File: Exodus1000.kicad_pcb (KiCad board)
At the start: 2 copper layers, 81.3 x 132.1 mm, 35 parts, among them J1 ARJ-169, M1 ET60S-02-24-02-X-VP-GP, M2 ET60S-02-24-02-X-VP-GP, M3 ET60S-02-24-02-X-VP-GP, M4 ET60S-02-24-02-X-VP-GP, U1 TM4C1294NCPDTGOOD, U2 93LCxxB, U3 FT232H, U4 TUSB4041I, U5 FSUSB42UMX, Y1 Crystal_GND24, Y2 Crystal

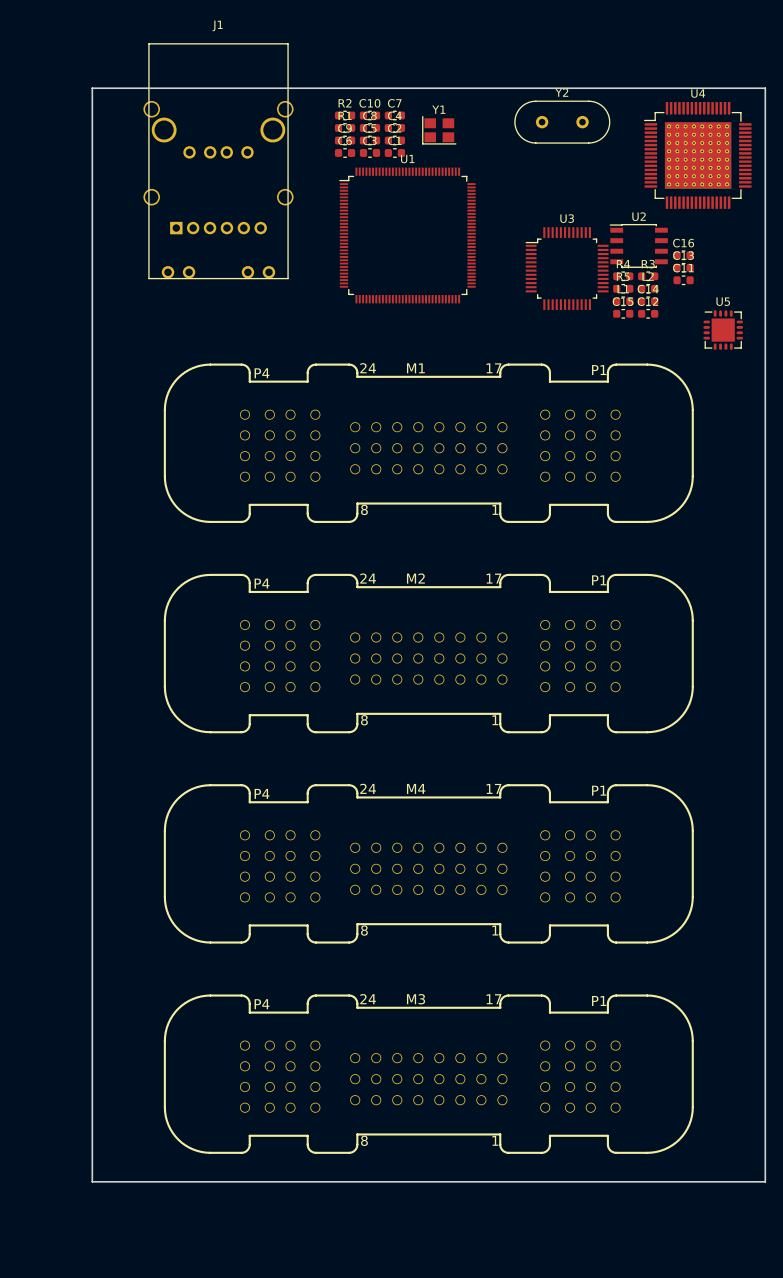
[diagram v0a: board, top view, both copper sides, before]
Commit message: layout stuff
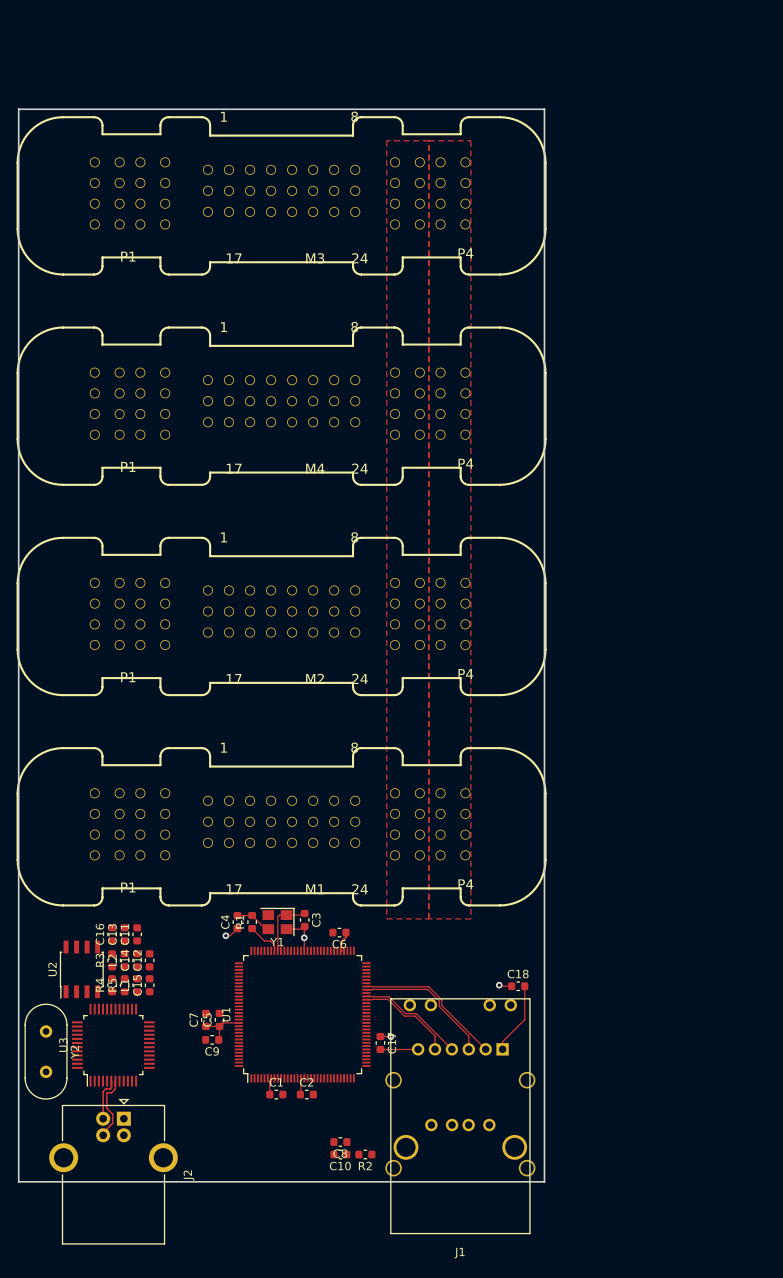
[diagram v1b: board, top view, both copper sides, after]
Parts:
- removed U4: TUSB4041I, Package_QFP:HTQFP-64-1EP_10x10mm_P0.5mm_EP8x8mm_Mask4.4x4.4mm_ThermalVias
- removed U5: FSUSB42UMX, Package_DFN_QFN:MLPQ-16-1EP_4x4mm_P0.65mm_EP2.8x2.8mm
- added C17: C_Small, Capacitor_SMD:C_0603_1608Metric, F.Cu at (118.6, 140.7)
- added C18: C_Small, Capacitor_SMD:C_0603_1608Metric, F.Cu at (135.3, 133.9)
- added J2: USB_B, Connector_USB:USB_B_OST_USB-B1HSxx_Horizontal, F.Cu at (87.6, 149.9)
- moved J1 131.2 mm to (128.3, 155.8), turned to 0 degrees
- moved C10 125.5 mm to (113.8, 154.2), turned to 180 degrees
- moved R2 125.5 mm to (116.8, 154.2), turned to 180 degrees
- moved Y2 125.1 mm to (78.2, 139.3), turned to 270 degrees
- moved C8 122.5 mm to (113.8, 152.7), turned to 180 degrees
- moved C2 115.7 mm to (109.7, 146.9)
- moved C1 114.6 mm to (106.0, 146.9)
- moved C7 111.6 mm to (97.5, 137.9), turned to 90 degrees
- moved U2 110.3 mm to (82.5, 131.8), turned to 90 degrees
- moved C9 109.8 mm to (98.3, 140.3), turned to 180 degrees
- moved U3 108.6 mm to (86.4, 141.0), turned to 90 degrees
- moved M3 108.2 mm to (106.7, 38.1), turned to 180 degrees
- moved C5 107.7 mm to (99.2, 137.9), turned to 90 degrees
- moved C16 107.2 mm to (86.2, 127.6), turned to 90 degrees
- moved R4 105.6 mm to (86.2, 133.7), turned to 90 degrees
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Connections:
- J1 pad P2: Net-(J1-PadP2) -> /TM4C129/ETH_TXO_P
- J1 pad P3: Net-(J1-PadP3) -> /TM4C129/ETH_TXO_N
- J1 pad P4: Net-(J1-PadP4) -> /TM4C129/ETH_RXI_P
- J1 pad P5: Net-(J1-PadP5) -> /TM4C129/ETH_RXI_N
- J1 pad SH1: Net-(J1-PadSH1) -> GND
- J1 pad SH2: Net-(J1-PadSH1) -> GND
- J1 pad SH3: Net-(J1-PadSH1) -> GND
- J1 pad SH4: Net-(J1-PadSH1) -> GND
- J1 pad SH5: Net-(J1-PadSH1) -> GND
- J1 pad SH6: Net-(J1-PadSH1) -> GND
- J1 pad U2: Net-(J1-PadU2) -> /TM4C129/USB_D_N
- J1 pad U3: Net-(J1-PadU3) -> /TM4C129/USB_D_P
- J1 pad U4: Net-(J1-PadU4) -> GND
- M1 pad P1-1: Net-(M1-PadP1-1) -> GND
- M1 pad P1-2: Net-(M1-PadP1-2) -> GND
- M1 pad P1-3: Net-(M1-PadP1-3) -> GND
- M1 pad P1-4: Net-(M1-PadP1-4) -> GND
- M1 pad P1-5: Net-(M1-PadP1-5) -> GND
- M1 pad P1-6: Net-(M1-PadP1-6) -> GND
- M1 pad P1-7: Net-(M1-PadP1-7) -> GND
- M1 pad P1-8: Net-(M1-PadP1-8) -> GND
- M1 pad P2-1: Net-(M1-PadP2-1) -> +BATT
- M1 pad P2-2: Net-(M1-PadP2-2) -> +BATT
- M1 pad P2-3: Net-(M1-PadP2-3) -> +BATT
- M1 pad P2-4: Net-(M1-PadP2-4) -> +BATT
- M1 pad P2-5: Net-(M1-PadP2-5) -> +BATT
- M1 pad P2-6: Net-(M1-PadP2-6) -> +BATT
- M1 pad P2-7: Net-(M1-PadP2-7) -> +BATT
- M1 pad P2-8: Net-(M1-PadP2-8) -> +BATT
- M1 pad P3-1: Net-(M1-PadP3-1) -> +5V
- M1 pad P3-2: Net-(M1-PadP3-2) -> +5V
- M1 pad P3-3: Net-(M1-PadP3-3) -> +5V
- M1 pad P3-4: Net-(M1-PadP3-4) -> +5V
- M1 pad P3-5: Net-(M1-PadP3-5) -> +5V
- M1 pad P3-6: Net-(M1-PadP3-6) -> +5V
- M1 pad P3-7: Net-(M1-PadP3-7) -> +5V
- M1 pad P3-8: Net-(M1-PadP3-8) -> +5V
- M1 pad P4-1: Net-(M1-PadP4-1) -> +3V3
- M1 pad P4-2: Net-(M1-PadP4-2) -> +3V3
- M1 pad P4-3: Net-(M1-PadP4-3) -> +3V3
- M1 pad P4-4: Net-(M1-PadP4-4) -> +3V3
- M1 pad P4-5: Net-(M1-PadP4-5) -> +3V3
- M1 pad P4-6: Net-(M1-PadP4-6) -> +3V3
- M1 pad P4-7: Net-(M1-PadP4-7) -> +3V3
- M1 pad P4-8: Net-(M1-PadP4-8) -> +3V3
- M2 pad P1-1: Net-(M2-PadP1-1) -> GND
- M2 pad P1-2: Net-(M2-PadP1-2) -> GND
- M2 pad P1-3: Net-(M2-PadP1-3) -> GND
- M2 pad P1-4: Net-(M2-PadP1-4) -> GND
- M2 pad P1-5: Net-(M2-PadP1-5) -> GND
- M2 pad P1-6: Net-(M2-PadP1-6) -> GND
- M2 pad P1-7: Net-(M2-PadP1-7) -> GND
- M2 pad P1-8: Net-(M2-PadP1-8) -> GND
- M2 pad P2-1: Net-(M2-PadP2-1) -> +BATT
- M2 pad P2-2: Net-(M2-PadP2-2) -> +BATT
- M2 pad P2-3: Net-(M2-PadP2-3) -> +BATT
- M2 pad P2-4: Net-(M2-PadP2-4) -> +BATT
- M2 pad P2-5: Net-(M2-PadP2-5) -> +BATT
- M2 pad P2-6: Net-(M2-PadP2-6) -> +BATT
- M2 pad P2-7: Net-(M2-PadP2-7) -> +BATT
- M2 pad P2-8: Net-(M2-PadP2-8) -> +BATT
- M2 pad P3-1: Net-(M2-PadP3-1) -> +5V
- M2 pad P3-2: Net-(M2-PadP3-2) -> +5V
- M2 pad P3-3: Net-(M2-PadP3-3) -> +5V
- M2 pad P3-4: Net-(M2-PadP3-4) -> +5V
- M2 pad P3-5: Net-(M2-PadP3-5) -> +5V
- M2 pad P3-6: Net-(M2-PadP3-6) -> +5V
- M2 pad P3-7: Net-(M2-PadP3-7) -> +5V
- M2 pad P3-8: Net-(M2-PadP3-8) -> +5V
- M2 pad P4-1: Net-(M2-PadP4-1) -> +3V3
- M2 pad P4-2: Net-(M2-PadP4-2) -> +3V3
- M2 pad P4-3: Net-(M2-PadP4-3) -> +3V3
- M2 pad P4-4: Net-(M2-PadP4-4) -> +3V3
- M2 pad P4-5: Net-(M2-PadP4-5) -> +3V3
- M2 pad P4-6: Net-(M2-PadP4-6) -> +3V3
- M2 pad P4-7: Net-(M2-PadP4-7) -> +3V3
- M2 pad P4-8: Net-(M2-PadP4-8) -> +3V3
- M3 pad P1-1: Net-(M3-PadP1-1) -> GND
- M3 pad P1-2: Net-(M3-PadP1-2) -> GND
- M3 pad P1-3: Net-(M3-PadP1-3) -> GND
- M3 pad P1-4: Net-(M3-PadP1-4) -> GND
- M3 pad P1-5: Net-(M3-PadP1-5) -> GND
- M3 pad P1-6: Net-(M3-PadP1-6) -> GND
- M3 pad P1-7: Net-(M3-PadP1-7) -> GND
- M3 pad P1-8: Net-(M3-PadP1-8) -> GND
- M3 pad P2-1: Net-(M3-PadP2-1) -> +BATT
- M3 pad P2-2: Net-(M3-PadP2-2) -> +BATT
- M3 pad P2-3: Net-(M3-PadP2-3) -> +BATT
- M3 pad P2-4: Net-(M3-PadP2-4) -> +BATT
- M3 pad P2-5: Net-(M3-PadP2-5) -> +BATT
- M3 pad P2-6: Net-(M3-PadP2-6) -> +BATT
- M3 pad P2-7: Net-(M3-PadP2-7) -> +BATT
- M3 pad P2-8: Net-(M3-PadP2-8) -> +BATT
- M3 pad P3-1: Net-(M3-PadP3-1) -> +5V
- M3 pad P3-2: Net-(M3-PadP3-2) -> +5V
- M3 pad P3-3: Net-(M3-PadP3-3) -> +5V
- M3 pad P3-4: Net-(M3-PadP3-4) -> +5V
- M3 pad P3-5: Net-(M3-PadP3-5) -> +5V
- M3 pad P3-6: Net-(M3-PadP3-6) -> +5V
- M3 pad P3-7: Net-(M3-PadP3-7) -> +5V
- M3 pad P3-8: Net-(M3-PadP3-8) -> +5V
- M3 pad P4-1: Net-(M3-PadP4-1) -> +3V3
- M3 pad P4-2: Net-(M3-PadP4-2) -> +3V3
- M3 pad P4-3: Net-(M3-PadP4-3) -> +3V3
- M3 pad P4-4: Net-(M3-PadP4-4) -> +3V3
- M3 pad P4-5: Net-(M3-PadP4-5) -> +3V3
- M3 pad P4-6: Net-(M3-PadP4-6) -> +3V3
- M3 pad P4-7: Net-(M3-PadP4-7) -> +3V3
- M3 pad P4-8: Net-(M3-PadP4-8) -> +3V3
- M4 pad P1-1: Net-(M4-PadP1-1) -> GND
- M4 pad P1-2: Net-(M4-PadP1-2) -> GND
- M4 pad P1-3: Net-(M4-PadP1-3) -> GND
- M4 pad P1-4: Net-(M4-PadP1-4) -> GND
- M4 pad P1-5: Net-(M4-PadP1-5) -> GND
- M4 pad P1-6: Net-(M4-PadP1-6) -> GND
- M4 pad P1-7: Net-(M4-PadP1-7) -> GND
- M4 pad P1-8: Net-(M4-PadP1-8) -> GND
- M4 pad P2-1: Net-(M4-PadP2-1) -> +BATT
- M4 pad P2-2: Net-(M4-PadP2-2) -> +BATT
- M4 pad P2-3: Net-(M4-PadP2-3) -> +BATT
- M4 pad P2-4: Net-(M4-PadP2-4) -> +BATT
- M4 pad P2-5: Net-(M4-PadP2-5) -> +BATT
- M4 pad P2-6: Net-(M4-PadP2-6) -> +BATT
- M4 pad P2-7: Net-(M4-PadP2-7) -> +BATT
- M4 pad P2-8: Net-(M4-PadP2-8) -> +BATT
- M4 pad P3-1: Net-(M4-PadP3-1) -> +5V
- M4 pad P3-2: Net-(M4-PadP3-2) -> +5V
- M4 pad P3-3: Net-(M4-PadP3-3) -> +5V
- M4 pad P3-4: Net-(M4-PadP3-4) -> +5V
- M4 pad P3-5: Net-(M4-PadP3-5) -> +5V
- M4 pad P3-6: Net-(M4-PadP3-6) -> +5V
- M4 pad P3-7: Net-(M4-PadP3-7) -> +5V
- M4 pad P3-8: Net-(M4-PadP3-8) -> +5V
- M4 pad P4-1: Net-(M4-PadP4-1) -> +3V3
- M4 pad P4-2: Net-(M4-PadP4-2) -> +3V3
- M4 pad P4-3: Net-(M4-PadP4-3) -> +3V3
- M4 pad P4-4: Net-(M4-PadP4-4) -> +3V3
- M4 pad P4-5: Net-(M4-PadP4-5) -> +3V3
- M4 pad P4-6: Net-(M4-PadP4-6) -> +3V3
- M4 pad P4-7: Net-(M4-PadP4-7) -> +3V3
- M4 pad P4-8: Net-(M4-PadP4-8) -> +3V3
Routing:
- net /TM4C129/ETH_TXO_P: track 0.00 -> 18.0 mm
- net /TM4C129/ETH_TXO_N: track 0.00 -> 16.7 mm
- net /TM4C129/ETH_RXI_P: track 0.00 -> 13.0 mm
- net /TM4C129/ETH_RXI_N: track 0.00 -> 11.8 mm
- net GND: track 0.00 -> 9.88 mm, vias 0 -> 4
- net Net-(C18-Pad2): track 0.00 -> 8.73 mm
- net /ft232h/D+: track 0.00 -> 8.05 mm
- net +3V3: track 0.00 -> 7.66 mm
- net /TM4C129/OSC0: track 0.00 -> 7.54 mm
- net Net-(C5-Pad1): track 0.00 -> 5.83 mm
- net /ft232h/D-: track 0.00 -> 5.28 mm
- net Net-(C17-Pad2): track 0.00 -> 4.56 mm
- net Net-(C4-Pad2): track 0.00 -> 4.40 mm
- net /TM4C129/OSC1: track 0.00 -> 4.23 mm
- added copper zone on F.Cu, net +3V3
- added copper zone on F.Cu, net +5V
- added copper zone on In1.Cu, net +BATT
- added copper zone on In2.Cu, net GND
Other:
- board size 81.3 x 132.1 mm -> 63.5 x 129.5 mm
- copper layers 2 -> 4
- rule trace_min: 0.2 -> 0.127
- rule via_min_drill: 0.3 -> 0.254
- rule via_min_size: 0.4 -> 0.508
